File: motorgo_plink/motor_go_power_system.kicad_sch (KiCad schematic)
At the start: 21 parts, among them U11 HUSB238_002DD, U7 AMS1117-3.3, U9 TPS54620RHLR

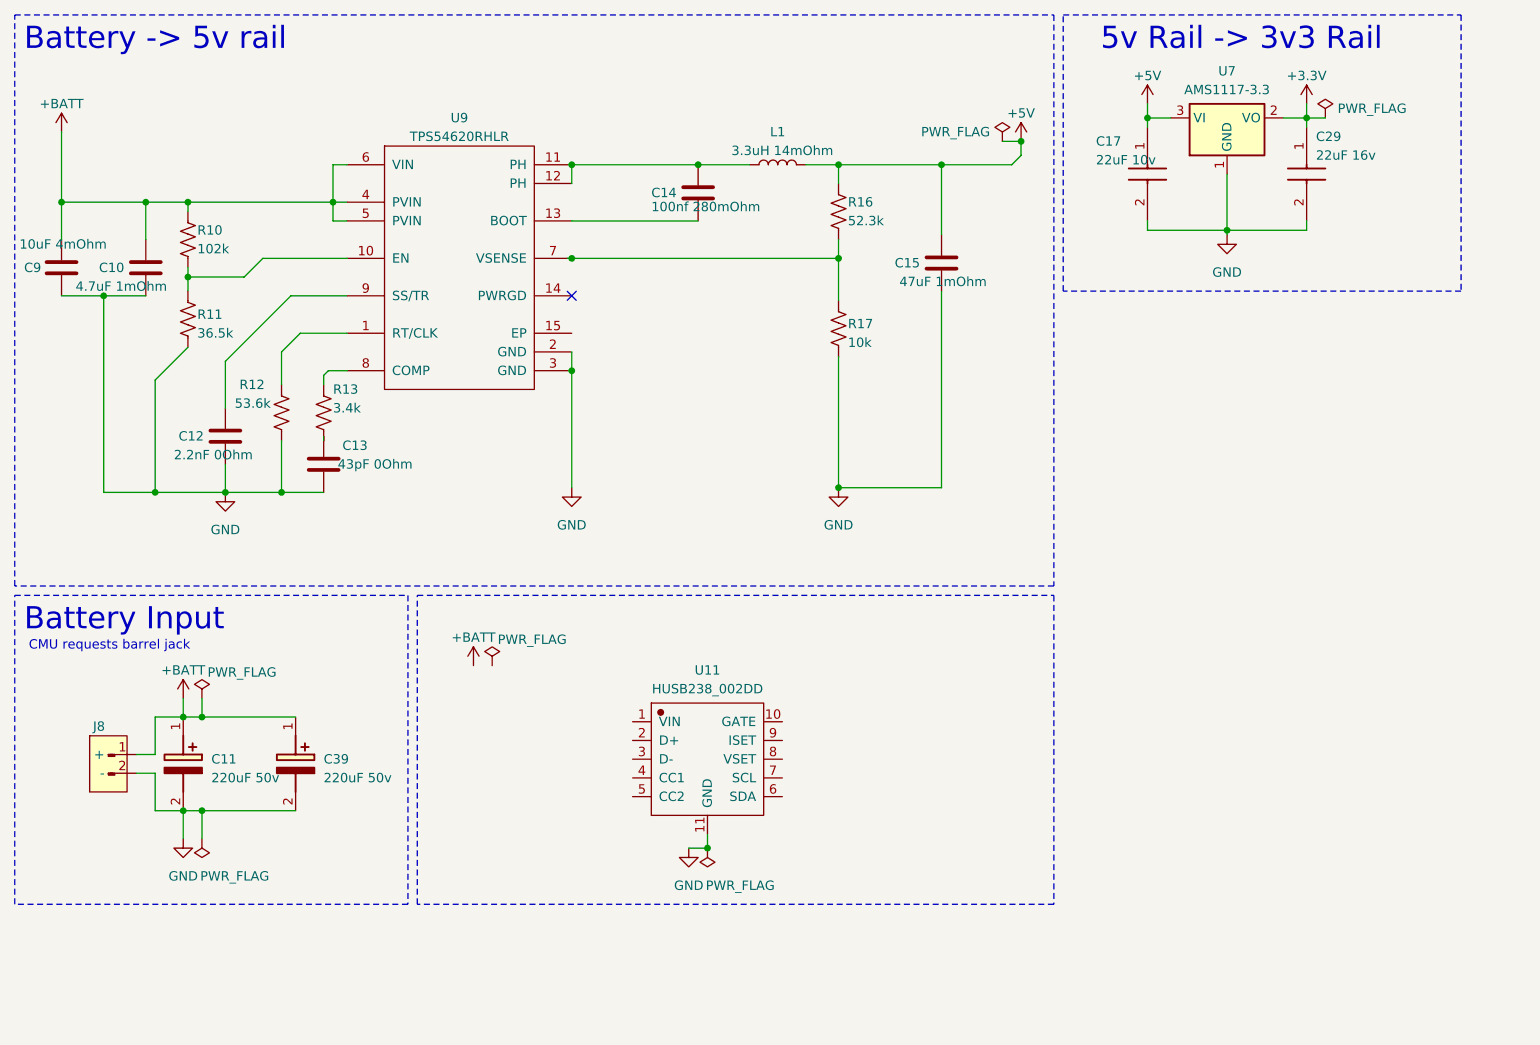
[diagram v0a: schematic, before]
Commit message: WIP update, schematic mainly complete
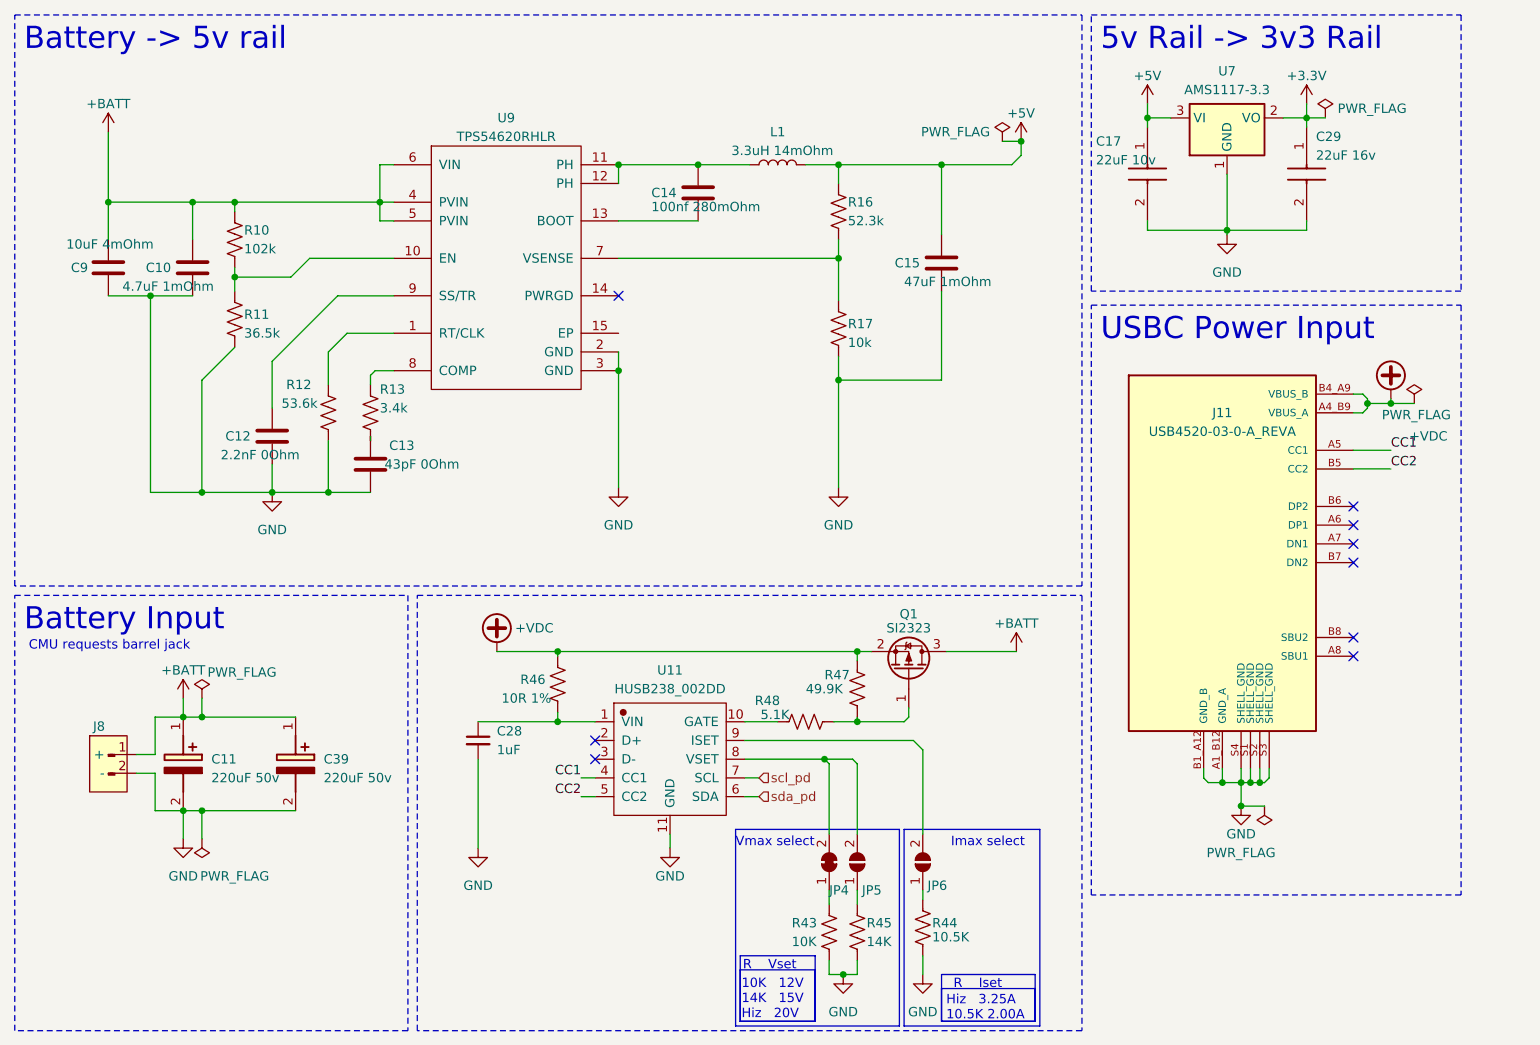
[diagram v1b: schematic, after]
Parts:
- added C28: 1uF, symbol Device:C_Small
- added J11: USB4520-03-0-A_REVA, aaa_motorgo_components:GCT_USB4520-03-0-A_REVA, symbol USB4520-03-0-A_REVA:USB4520-03-0-A_REVA
- added JP4: SolderJumper_2_Bridged, symbol Jumper:SolderJumper_2_Bridged
- added JP5, JP6: SolderJumper_2_Open, symbol Jumper:SolderJumper_2_Open
- added Q1: SI2323, symbol Device:Q_PMOS_GSD
- added R43: 10K, symbol Device:R_US
- added R44: 10.5K, symbol Device:R_US
- added R45: 14K, symbol Device:R_US
- added R46: 10R 1%, symbol Device:R_US
- added R47: 49.9K, symbol Device:R_US
- added R48: 5.1K, symbol Device:R_US
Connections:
- net +BATT: now also Q1.3 (D)
- net GND: now also C28.2, J11.A1_B12 (GND_A), J11.B1_A12 (GND_B), J11.S1 (SHELL_GND), J11.S2 (SHELL_GND), J11.S3 (SHELL_GND), J11.S4 (SHELL_GND), R43.2, R44.2, R45.2
- net at U11.1 (VIN): now also C28.1, R46.2
- net at U11.10 (GATE): now also R48.1
- net CC1: now reaches U11.4 (CC1)
- net CC1: now also J11.A5 (CC1)
- net CC2: now reaches U11.5 (CC2)
- net CC2: now also J11.B5 (CC2)
- net sda_pd: now reaches U11.6 (SDA)
- net scl_pd: now reaches U11.7 (SCL)
- net at U11.8 (VSET): now also JP4.2 (B), JP5.2 (B)
- net at U11.9 (ISET): now also JP6.2 (B)
- new net: JP6.1 (A), R44.1
- new net: Q1.1 (G), R47.2, R48.2
- new net: JP4.1 (A), R43.1
- new net: JP5.1 (A), R45.1
- new net +VDC: J11.A4_B9 (VBUS_A), J11.B4_A9 (VBUS_B), Q1.2 (S), R46.1, R47.1
- no-connect marks 1 -> 9
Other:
- note added: "10K 12V 14K 15V Hiz 20V"
- note added: "Hiz 3.25A 10.5K 2.00A"
- note added: "Imax select"
- note added: "R Iset"
- note added: "R Vset"
- note added: "USBC Power Input"
- note added: "Vmax select"
- moved on the sheet: C10, C12, C13, C9, R10, R11, R12, R13, U11, U9
